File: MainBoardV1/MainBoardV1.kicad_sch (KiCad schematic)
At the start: 32 parts, among them J1 USB_B_Micro, J10 Conn_01x04, J2 Conn_01x04, J3 Conn_01x02, J4 Conn_01x04, J5 Conn_01x05, J6 Conn_01x02, J7 Conn_01x04, J8 Conn_01x04, J9 Conn_01x04, SW1 SW_SPST, SW2 SW_SPDT, SW3 SW_DIP_x03, SW4 SW_DIP_x03, SW5 SW_DIP_x03, U1 ESP32-S3-WROOM-1, U3 LM1117MP-3.3, U4 TEN20-2411WIN

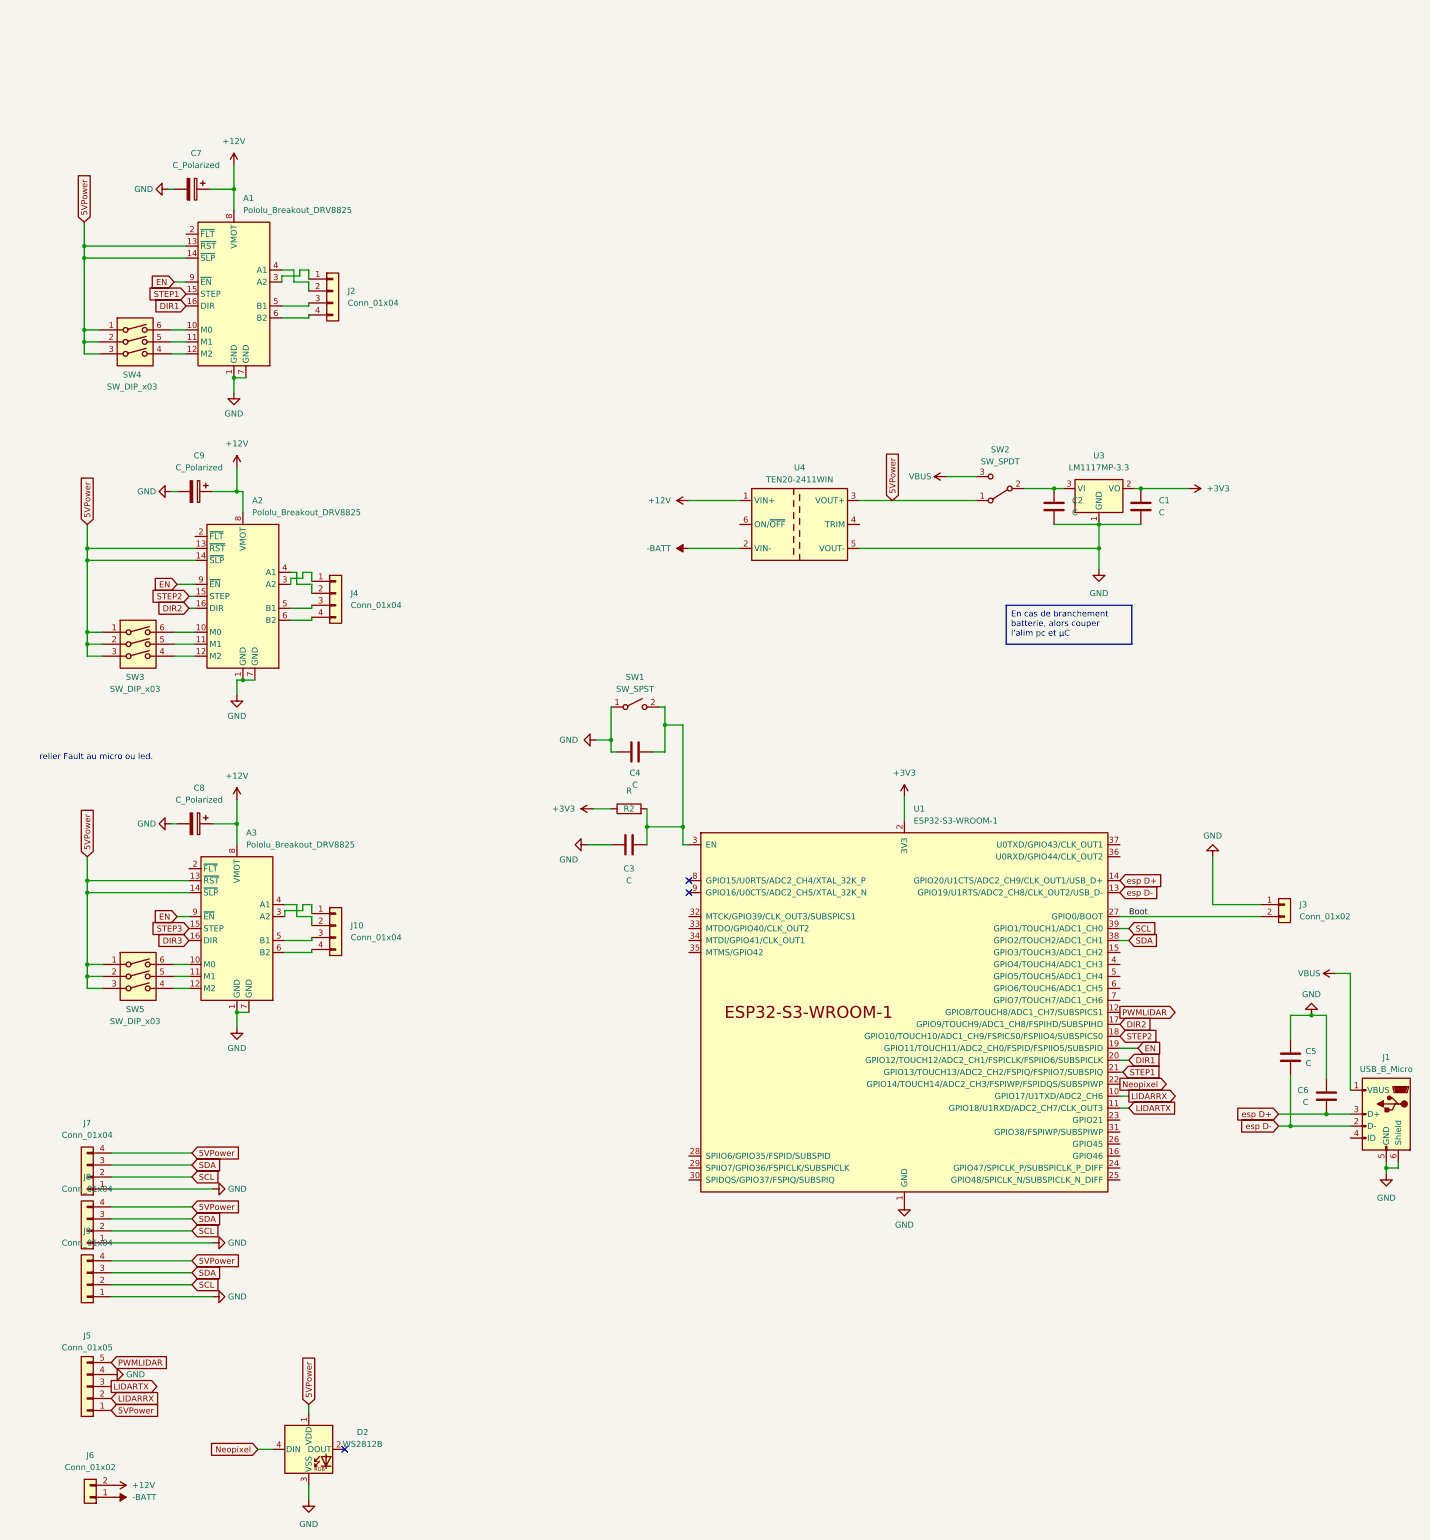
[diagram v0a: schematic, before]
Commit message: Merge of versions
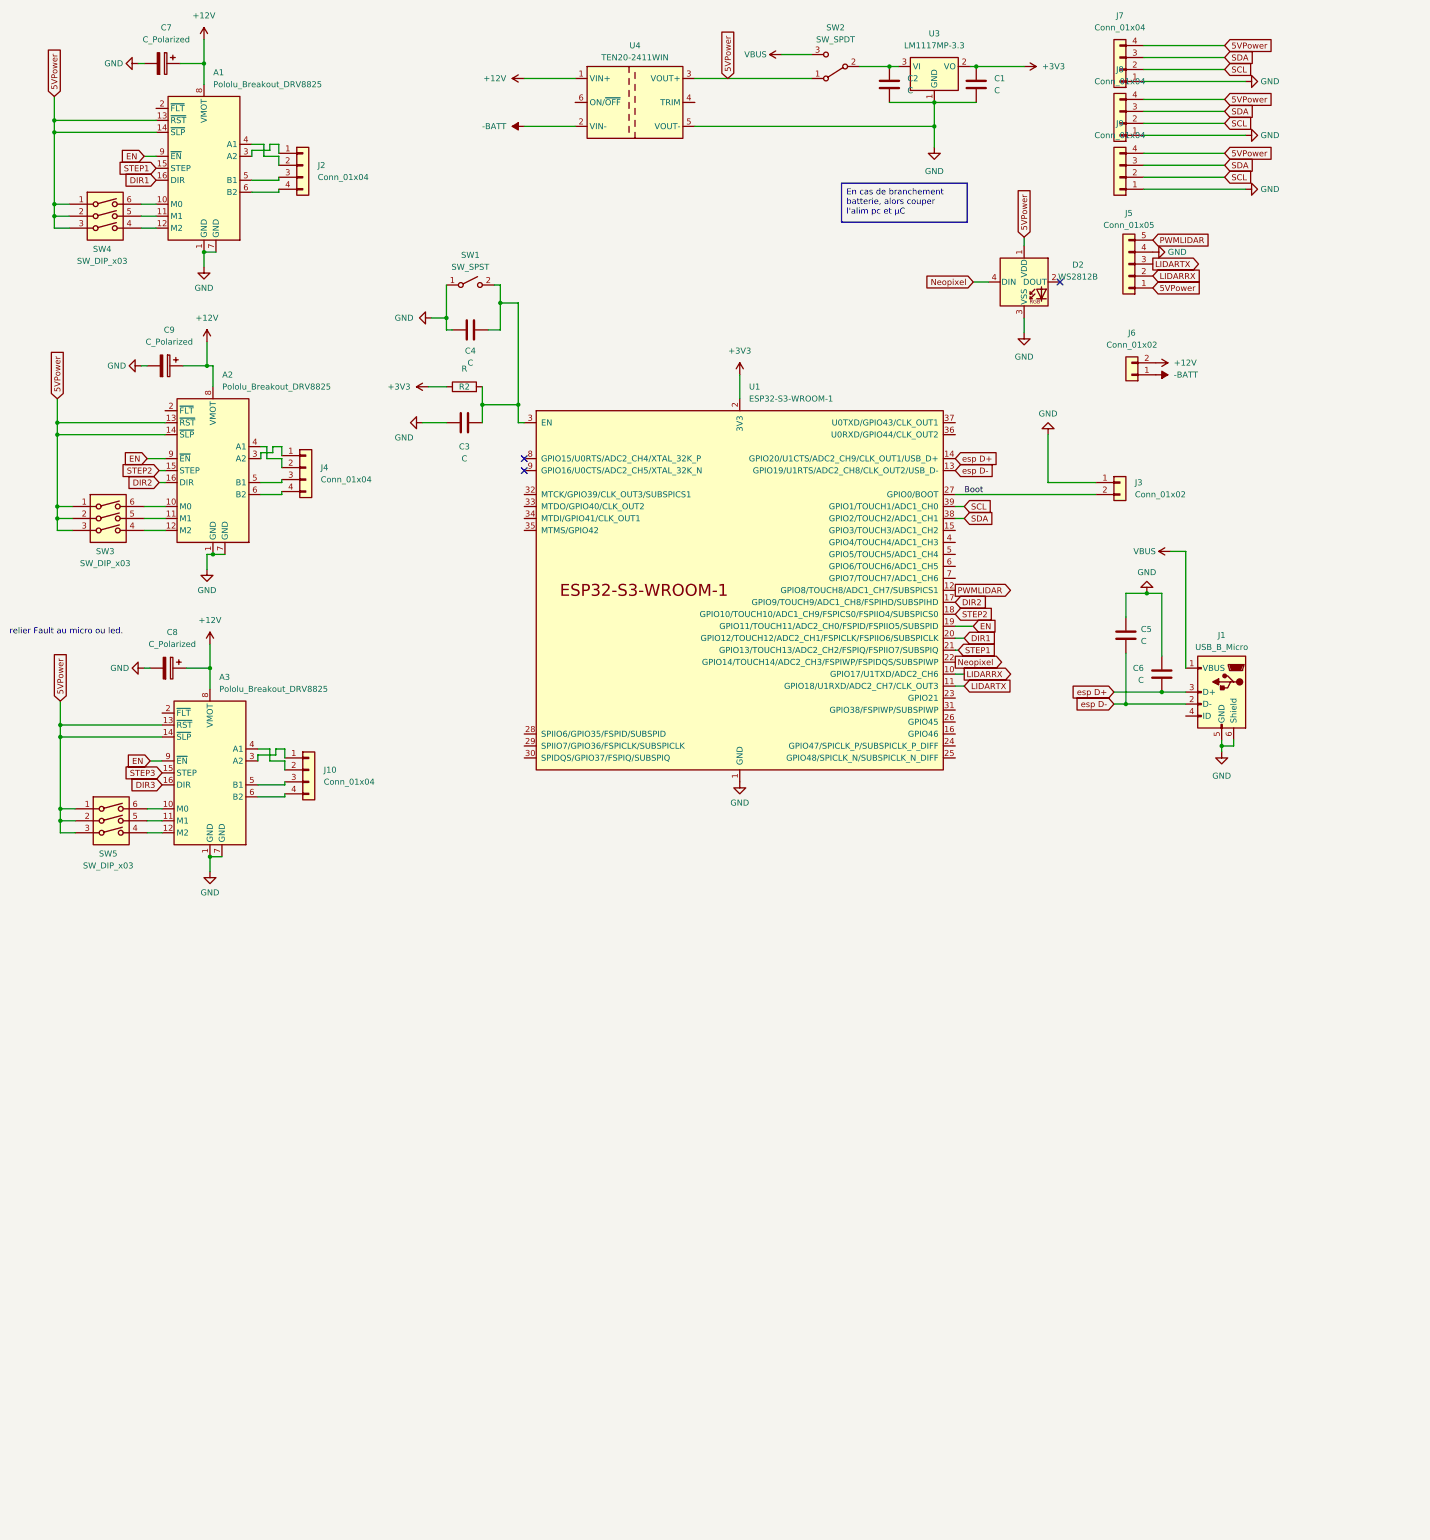
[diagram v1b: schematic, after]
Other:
- moved on the sheet: A1, A2, A3, C1, C2, C3, C4, C5, C6, C7, C8, C9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
